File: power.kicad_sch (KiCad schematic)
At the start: 32 parts, among them Q6 Q_PMOS_GDS, U10 AP6230xWU, U11 SIC463ED-T1-GE3, U12 AP6230xWU

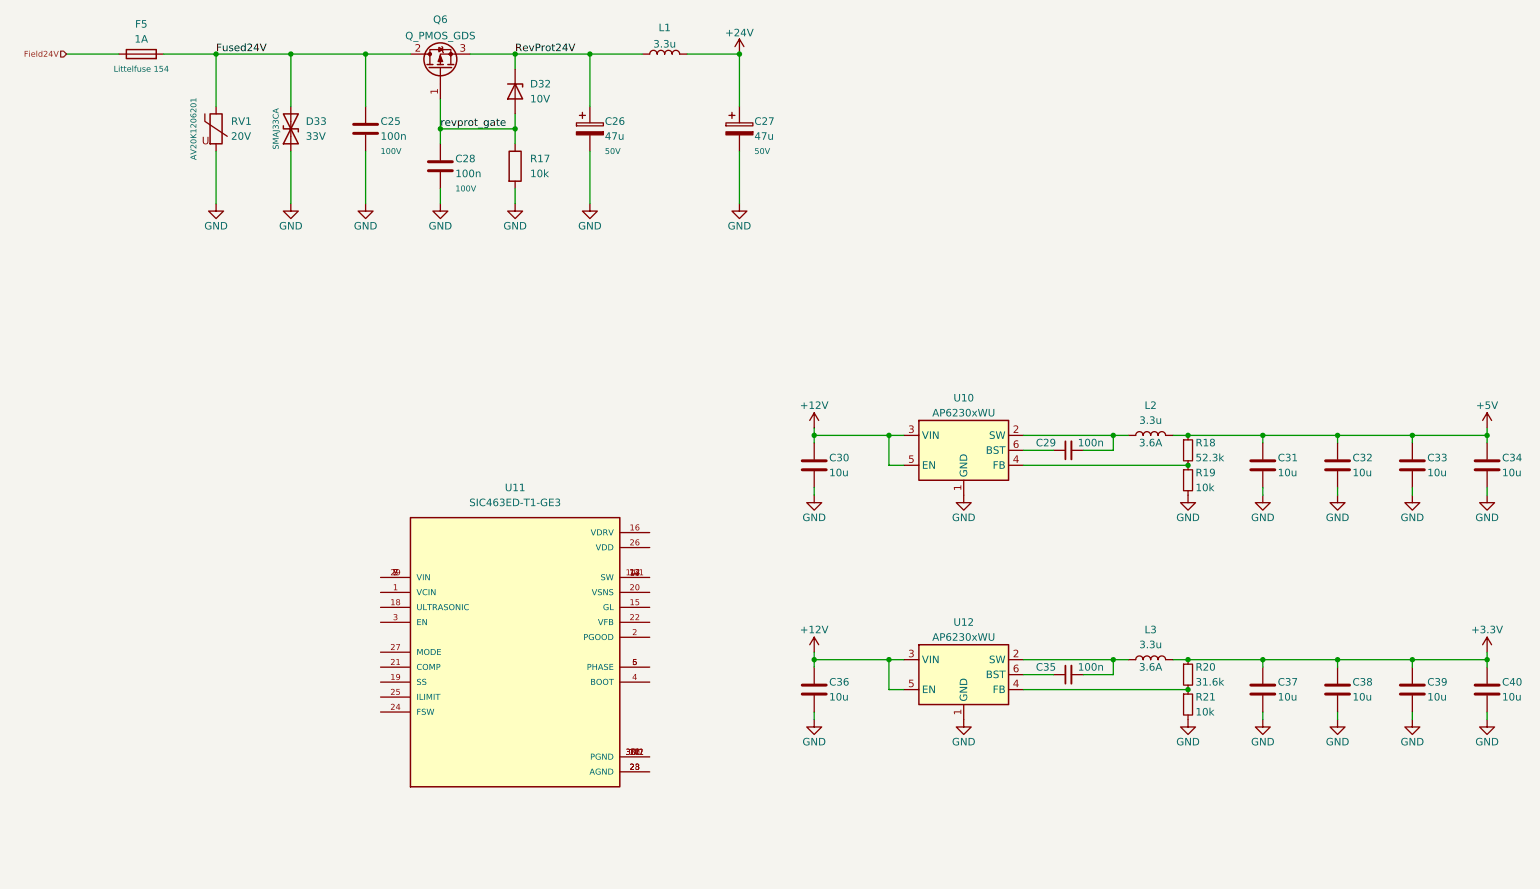
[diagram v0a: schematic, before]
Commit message: Done?
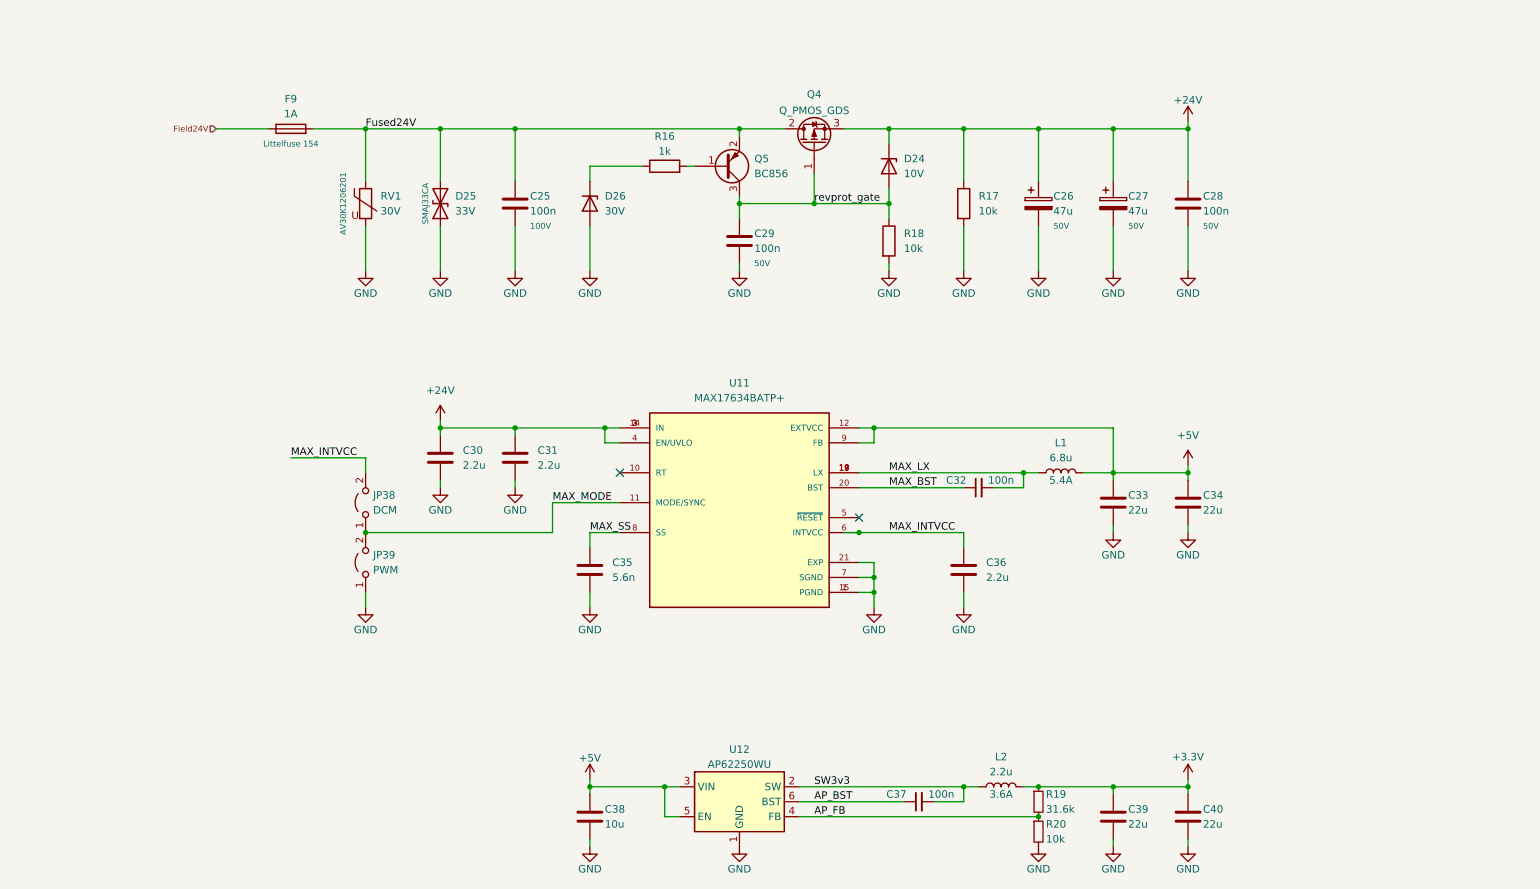
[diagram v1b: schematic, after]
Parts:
- removed C29: 100n, Capacitor_SMD:C_0603_1608Metric, symbol Device:C_Small
- removed C32, C39, C40: 10u, Capacitor_SMD:C_0805_2012Metric, symbol Device:C
- removed L2: 3.3u, symbol Device:L
- removed R18: 52.3k, Resistor_SMD:R_0603_1608Metric, symbol Device:R_Small
- removed R19: 10k, Resistor_SMD:R_0603_1608Metric, symbol Device:R_Small
- removed U10: AP6230xWU, Package_TO_SOT_SMD:SOT-23-6, symbol AP6230xWU:AP6230xWU
- removed U11: SIC463ED-T1-GE3, SIC463:CONV_SIC461ED-T1-GE3, symbol SIC461ED-T1-GE3:SIC461ED-T1-GE3
- added C28: 100n, Capacitor_SMD:C_0805_2012Metric, symbol Device:C
- added C32: 100n, Capacitor_SMD:C_0603_1608Metric, symbol Device:C_Small
- added C35: 5.6n, Capacitor_SMD:C_0603_1608Metric, symbol Device:C
- added C36: 2.2u, Capacitor_SMD:C_0603_1608Metric, symbol Device:C
- added D26: 30V, Diode_SMD:D_SOD-123, symbol Device:D_Zener
- added JP38: DCM, Jumper:SolderJumper-2_P1.3mm_Open_TrianglePad1.0x1.5mm, symbol Jumper:Jumper_2_Open
- added JP39: PWM, Jumper:SolderJumper-2_P1.3mm_Open_TrianglePad1.0x1.5mm, symbol Jumper:Jumper_2_Open
- added Q5: BC856, Package_TO_SOT_SMD:SOT-23, symbol Transistor_BJT:BC856
- added R16: 1k, Resistor_SMD:R_0603_1608Metric, symbol Device:R
- added R17: 10k, Resistor_SMD:R_0603_1608Metric, symbol Device:R
- added U11: MAX17634BATP+, MAX17634:TQFN20-EP, symbol MAX17634BATP_:MAX17634BATP+
- C29: renamed from C28; Voltage 100V -> 50V
- C30, C31: value 10u -> 2.2u; footprint Capacitor_SMD:C_0805_2012Metric -> Capacitor_SMD:C_1206_3216Metric
- C33, C34: value 10u -> 22u; footprint Capacitor_SMD:C_0805_2012Metric -> Capacitor_SMD:C_1206_3216Metric
- C39: renamed from C37; value 10u -> 22u; footprint Capacitor_SMD:C_0805_2012Metric -> Capacitor_SMD:C_1206_3216Metric
- C40: renamed from C38; value 10u -> 22u; footprint Capacitor_SMD:C_0805_2012Metric -> Capacitor_SMD:C_1206_3216Metric
- L1: value 3.3u -> 6.8u; footprint Inductor_SMD:L_1008_2520Metric -> Inductor_SMD:L_Abracon_ASPI-0630LR; Current (none) -> 5.4A
- L2: renamed from L3; value 3.3u -> 2.2u; footprint (none) -> Inductor_SMD:L_Taiyo-Yuden_NR-50xx
- RV1: value 20V -> 30V; Field4 AV20K1206201 -> AV30K1206201
- U12: value AP6230xWU -> AP62250WU; footprint Package_TO_SOT_SMD:SOT-23-6 -> TSOT26:TSOT26
- renumbered C35 to C37, C36 to C38, D32 to D24, D33 to D25, F5 to F9, Q6 to Q4, R17 to R18, R20 to R19, R21 to R20
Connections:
- net +24V: now also C26.1, C30.1, C31.1, D24.1 (K), Q4.3 (S), C28.1, R17.1, U11.14 (IN), U11.2 (IN), U11.3 (IN), U11.4 (EN/UVLO); no longer L1.2
- net +5V: now also C38.1, L1.2, U12.3 (VIN), U12.5 (EN), U11.12 (EXTVCC), U11.9 (FB); no longer C31.1
- net Fused24V: now also Q5.2 (E)
- net GND: now also C28.2, C35.2, C36.2, D26.2 (A), JP39.1 (A), R17.2, U11.1 (PGND), U11.15 (PGND), U11.21 (EXP), U11.7 (SGND)
- net revprot_gate: now also Q5.3 (C)
- net SW3v3: now reaches C37.2, L2.1, U12.2 (SW)
- net AP_FB: now reaches R19.2, R20.1, U12.4 (FB)
- net AP_BST: now reaches C37.1, U12.6 (BST)
- removed net +12V: C30.1, C38.1, U12.3 (VIN), U12.5 (EN)
- removed net RevProt24V: C26.1, D24.1 (K), L1.1, Q4.3 (S)
- new net: D26.1 (K), R16.1
- new net: Q5.1 (B), R16.2
- new net MAX_BST: C32.1, U11.20 (BST)
- new net MAX_INTVCC: C36.1, JP38.2 (B), U11.6 (INTVCC)
- new net MAX_LX: C32.2, L1.1, U11.17 (LX), U11.18 (LX), U11.19 (LX)
- new net MAX_MODE: JP38.1 (A), JP39.2 (B), U11.11 (MODE/SYNC)
- new net MAX_SS: C35.1, U11.8 (SS)
- no-connect marks 0 -> 2
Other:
- moved on the sheet: C25, C26, C27, C29, C37, C38, C39, C40, D24, D25, F9, L2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
